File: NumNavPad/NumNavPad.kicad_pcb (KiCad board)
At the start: 2 copper layers, 150.8 x 108 mm, 55 parts, among them U1 Elite-C

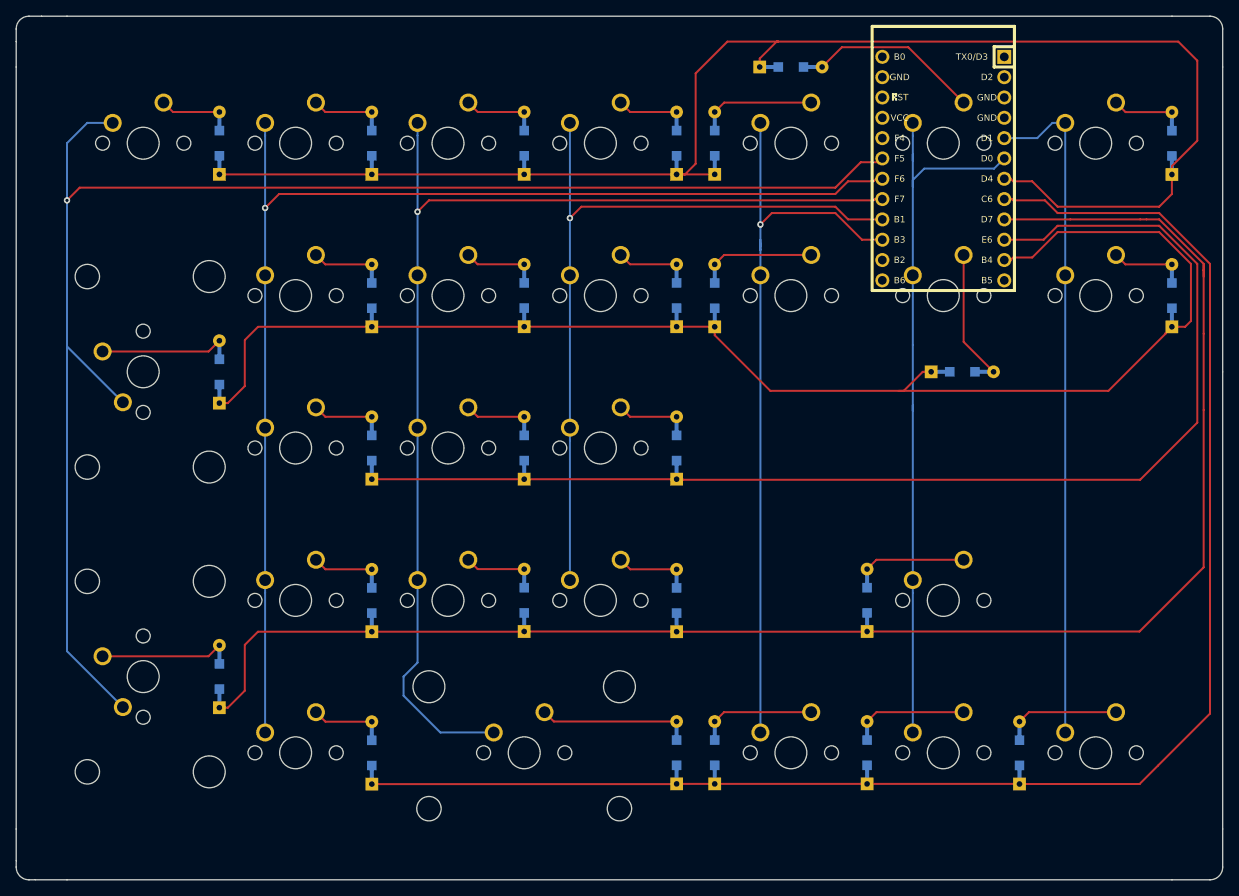
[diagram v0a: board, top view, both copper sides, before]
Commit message: Gerbers Added
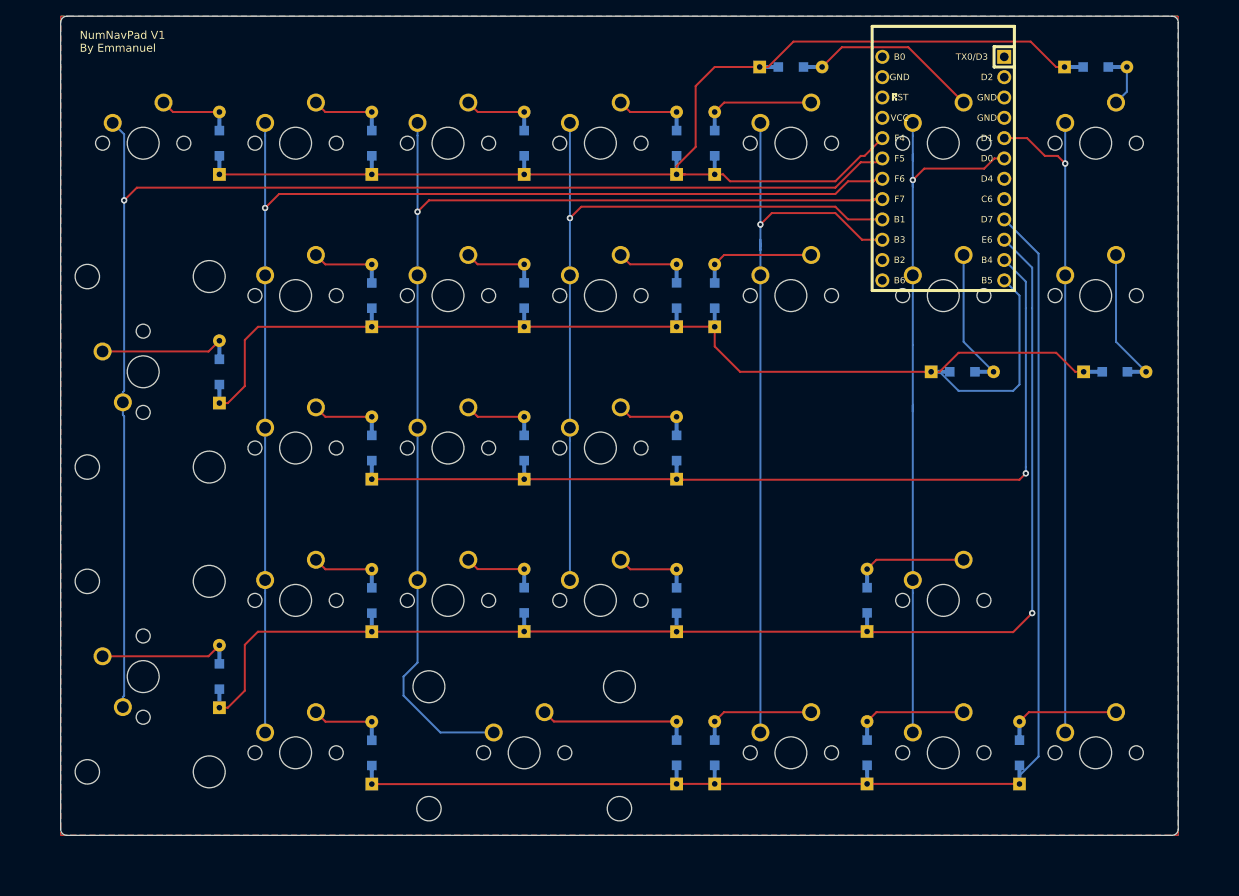
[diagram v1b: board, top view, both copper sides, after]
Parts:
- moved D7 13.5 mm to (161.9, 33.3), turned to 0 degrees
- moved D14 11.9 mm to (164.3, 71.4), turned to 0 degrees
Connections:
- U1 pad 10: Row2 -> Row3
- U1 pad 11: Row1 -> Row2
- U1 pad 12: Net-(U1-Pad12) -> Row1
- U1 pad 20: Net-(U1-Pad20) -> Row0
- U1 pad 7: Row0 -> Net-(U1-Pad7)
- U1 pad 8: Row4 -> Net-(U1-Pad8)
- U1 pad 9: Row3 -> Row4
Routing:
- net Row3: track 200.3 -> 158.1 mm, vias 0 -> 1
- net Row2: track 152.8 -> 111.5 mm, vias 0 -> 1
- net Row4: track 194.9 -> 155.5 mm
- net Row0: track 187.5 -> 148.7 mm
- net Row1: track 176.2 -> 147.3 mm
- net Col0: track 194.7 -> 171.4 mm
- net Net-(D14-Pad2): track 7.47 -> 16.2 mm
- net Net-(D7-Pad2): track 7.48 -> 5.01 mm
- net Net-(U1-Pad7): track 0.00 -> 1.55 mm
- net Col6: track 84.6 -> 85.1 mm, vias 0 -> 1
- net Col5: vias 0 -> 1
- added copper zone on B.Cu, net (none)
- added copper zone on F.Cu, net (none)
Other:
- board size 150.8 x 108 mm -> 139.7 x 102.4 mm
- board text added: "NumNavPad V1 By Emmanuel"
